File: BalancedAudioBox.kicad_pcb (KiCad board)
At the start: 2 copper layers, 90 x 72 mm, 66 parts, among them IC1 TPS61252DSGT, IC2 DRV135UA_2K5, IC3 DRV135UA_2K5, J1 Conn_02x10_Odd_Even, J2 Conn_01x03, J3 XLR3_Ground, J4 XLR3_Ground, J5 Conn_01x03, J6 Conn_01x02, J7 Conn_01x05, J8 Conn_01x03, U1 LM27762, U2 PCM5102

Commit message: adding regulator
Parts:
- R7: value 7k5 -> 2k2
- R8: value 2k7 -> 3k3
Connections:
- C1 pad 1: /PowerSupply/VIN -> VIN
- C27 pad 1: /PowerSupply/VIN -> VIN
- IC1 pad 6: /PowerSupply/VIN -> VIN
- IC1 pad 8: /PowerSupply/VIN -> VIN
- J2 pad 2: /PowerSupply/VIN -> VIN
- L1 pad 1: /PowerSupply/VIN -> VIN
- PS1 pad 1: /PowerSupply/VIN -> VIN
- R7 pad 1: +3V3 -> VIN

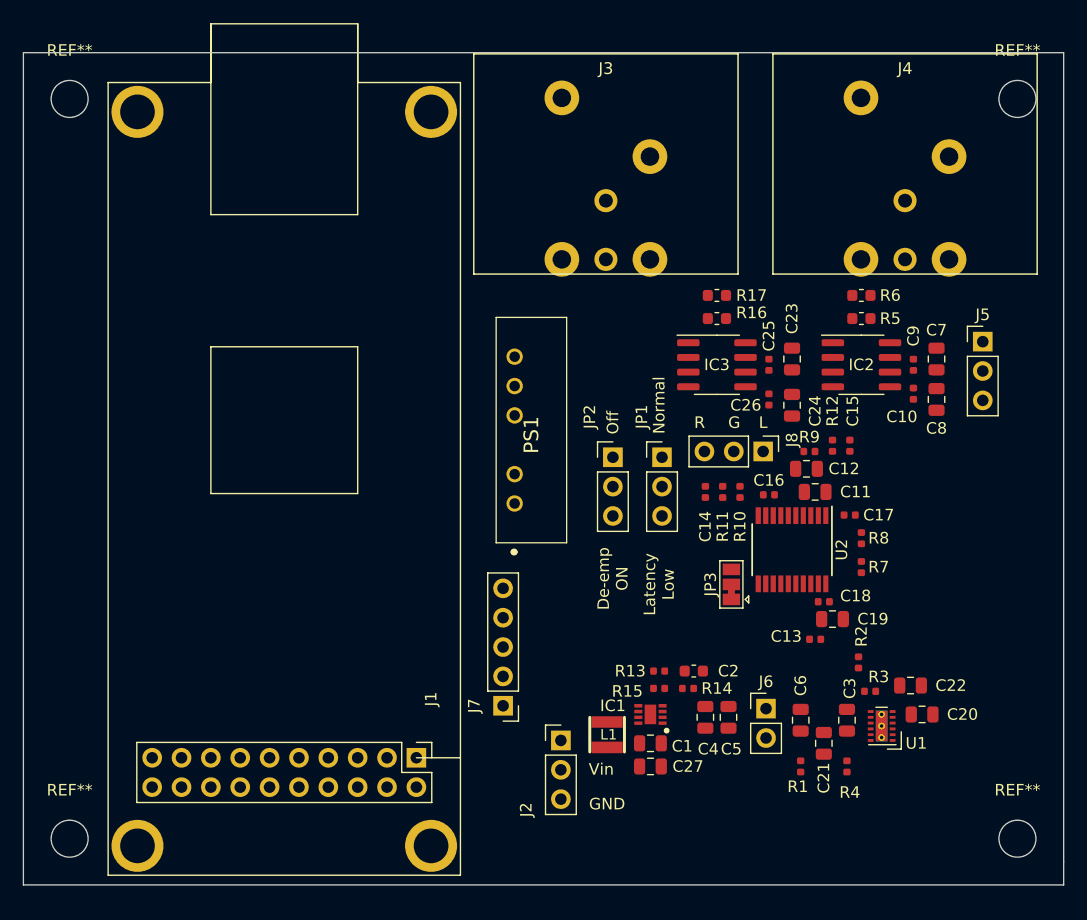
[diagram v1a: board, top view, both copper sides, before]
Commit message: more layout
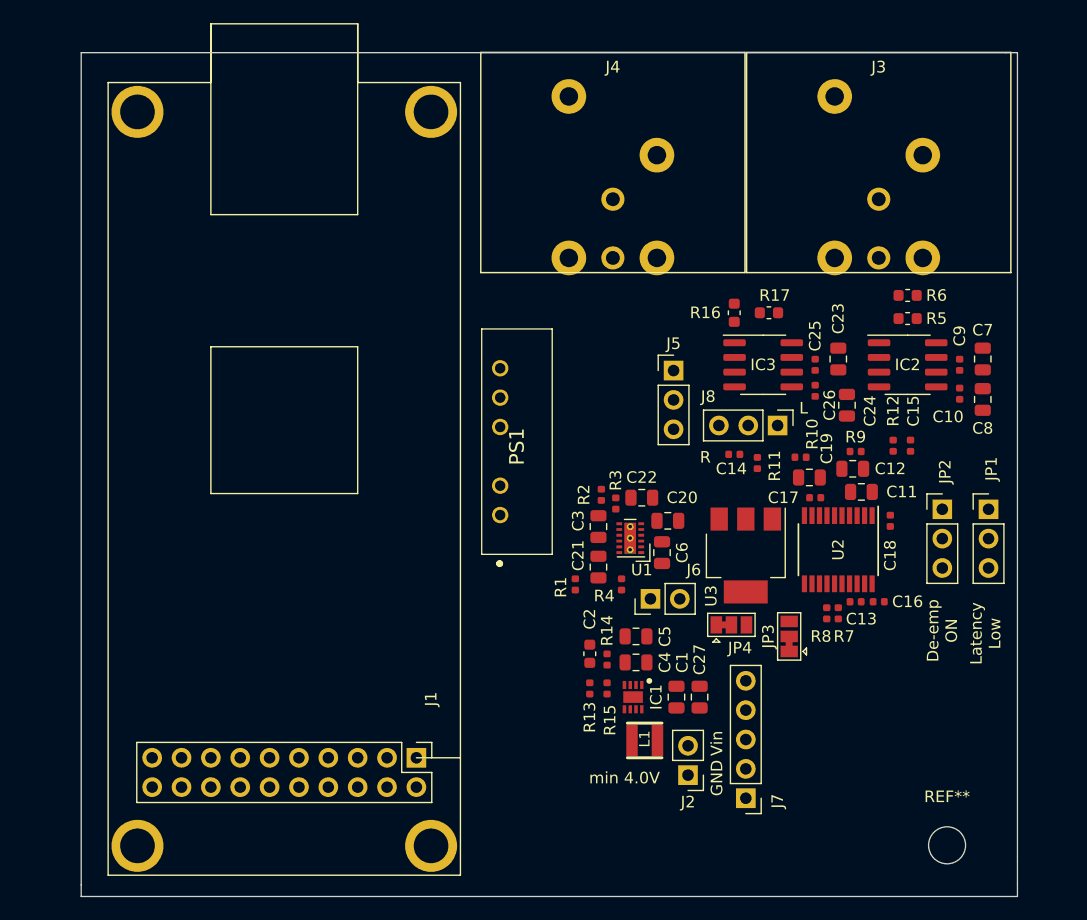
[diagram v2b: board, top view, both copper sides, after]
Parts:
- removed the REF** at (109.0, 131.0)
- removed the REF** at (109.0, 67.0)
- removed the REF** at (191.0, 67.0)
- added JP4: SolderJumper_3_Bridged12, Jumper:SolderJumper-3_P1.3mm_Bridged12_Pad1.0x1.5mm, F.Cu at (166.2, 112.5)
- added U3: AP1117-33, Package_TO_SOT_SMD:SOT-223-3_TabPin2, F.Cu at (167.5, 106.5)
- J2: value Conn_01x03 -> Conn_01x02; footprint Connector_PinHeader_2.54mm:PinHeader_1x03_P2.54mm_Vertical -> Connector_PinHeader_2.54mm:PinHeader_1x02_P2.54mm_Vertical
- moved JP2 28.9 mm to (184.5, 102.5)
- moved JP1 28.6 mm to (188.5, 102.5)
- moved C22 28.4 mm to (158.5, 101.5)
- moved C20 27.7 mm to (160.8, 103.5)
- moved R3 27.4 mm to (156.2, 102.0), turned to 270 degrees
- moved C3 27.3 mm to (154.8, 104.0)
- moved U1 27.2 mm to (157.5, 105.0)
- moved J5 26.9 mm to (161.2, 90.5)
- moved R2 26.6 mm to (155.0, 101.2)
- moved J4 25.3 mm to (156.0, 72.5)
- moved R1 25.1 mm to (152.8, 109.0)
- moved R4 25.1 mm to (156.8, 109.0)
- moved C21 24.8 mm to (154.8, 107.5), turned to 90 degrees
- moved J3 23.6 mm to (179.0, 72.5)
- moved J7 22.5 mm to (167.5, 127.5)
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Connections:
- net /PowerSupply/VOUT-5.4V renamed VOUT-5.4V
- C17 pad 1: +3V3 -> +3.3VA
- C18 pad 1: +3V3 -> +3.3VA
- C19 pad 1: +3V3 -> +3.3VA
- J2 pad 1: +3V3 -> GND
- U2 pad 1: +3V3 -> +3.3VA
- U2 pad 8: +3V3 -> +3.3VA
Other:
- board size 90 x 72 mm -> 81 x 73 mm
- board text added: "min 4.0V"
- board text removed: "G"
- board text removed: "Normal"
- board text removed: "Off"
